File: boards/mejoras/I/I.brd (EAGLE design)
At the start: 90 x 26 mm, 18 parts

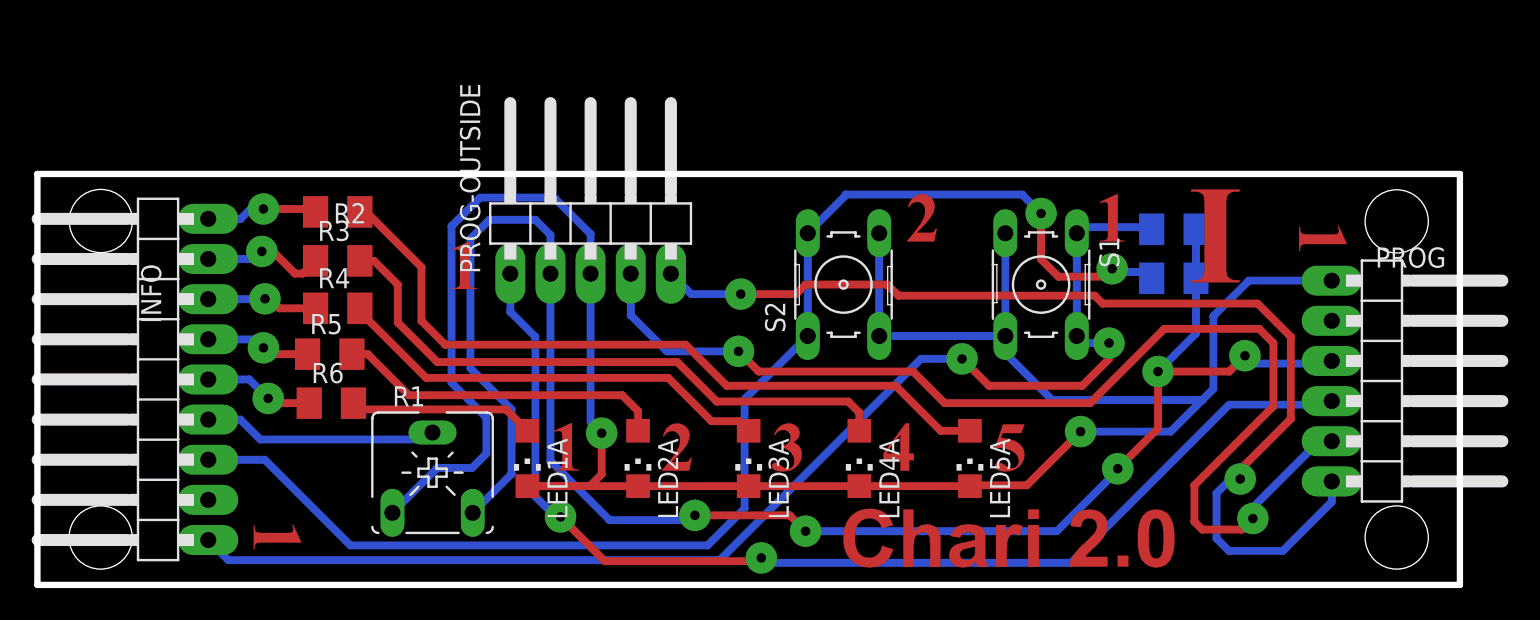
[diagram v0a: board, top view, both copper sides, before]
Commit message: updated board h and i
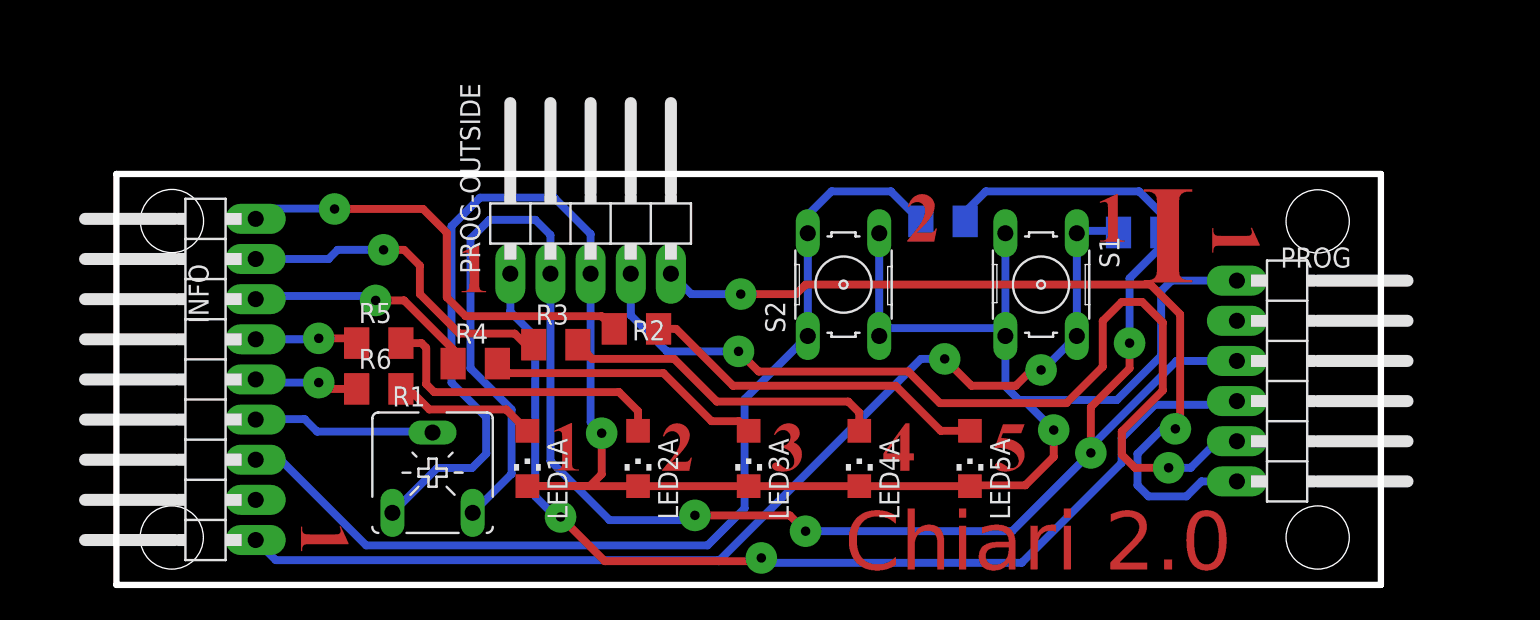
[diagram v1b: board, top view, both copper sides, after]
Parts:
- moved R2 20.3 mm to (37.9, 16.2)
- moved R8 15.0 mm to (57.3, 23.0)
- moved R3 14.8 mm to (32.8, 15.2)
- moved R4 9.38 mm to (27.7, 14.0)
- moved PROG 6.00 mm to (79.7, 12.9)
- moved R5 3.18 mm to (21.6, 15.3)
- moved R6 3.13 mm to (21.6, 12.4)
- moved INFO 3.00 mm to (10.0, 13.0)
- moved R7 2.11 mm to (69.8, 22.3)
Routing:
- net N$5: track 46.3 -> 22.4 mm
- net N$6: track 7.85 -> 28.5 mm
- net B2: track 83.3 -> 62.9 mm, vias 2 -> 0
- net N$4: track 38.8 -> 21.4 mm
- net N$7: track 7.90 -> 21.4 mm
- net PGC: track 66.6 -> 53.2 mm
- net 5V: track 108.9 -> 122.2 mm, vias 5 -> 4
- net PGD: track 72.9 -> 62.3 mm
- net GND: track 148.6 -> 138.1 mm
- net N$3: track 27.9 -> 17.7 mm
- net B1: track 79.0 -> 69.1 mm
- net N$8: track 7.05 -> 14.9 mm
- net MCRL: track 71.5 -> 66.4 mm
- net N$11: track 14.9 -> 11.6 mm
- net N$1: track 11.7 -> 9.10 mm
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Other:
- board size 90 x 26 mm -> 80 x 26 mm
